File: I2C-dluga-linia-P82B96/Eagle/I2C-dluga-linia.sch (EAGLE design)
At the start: 15 parts

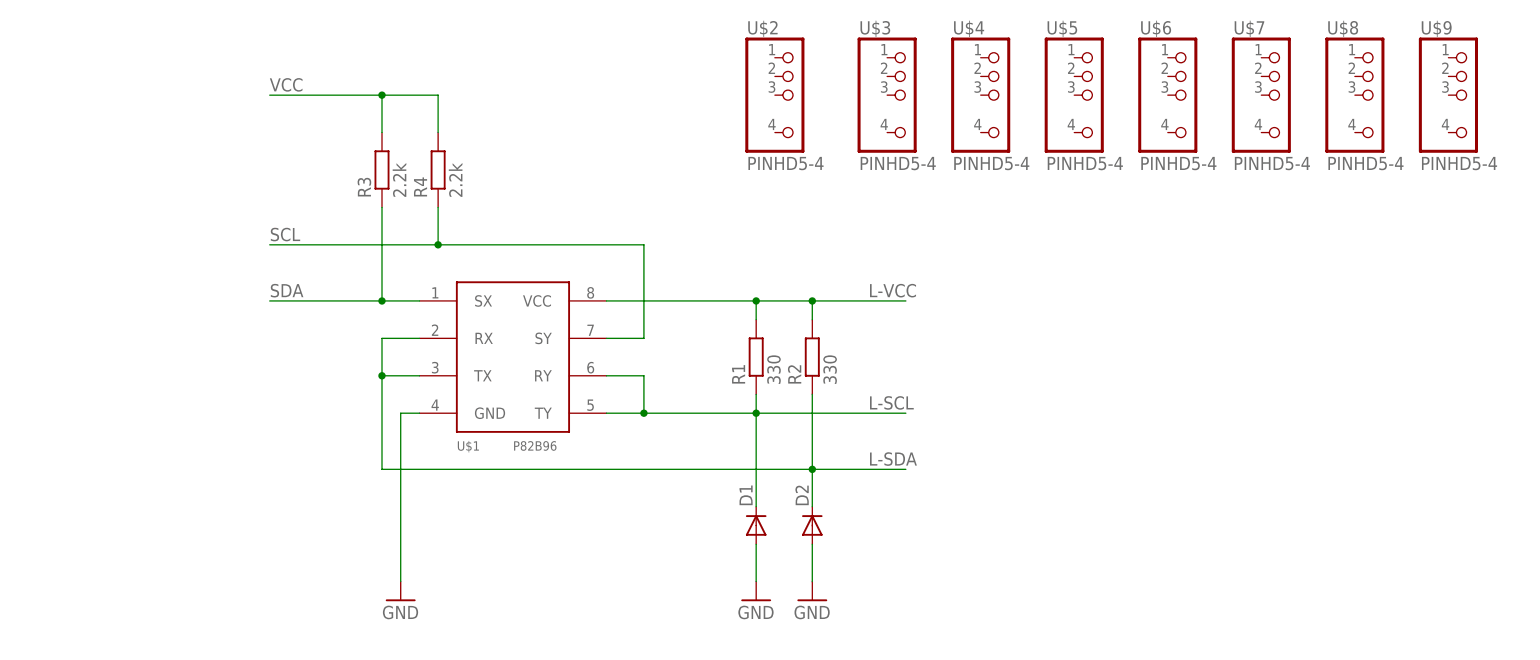
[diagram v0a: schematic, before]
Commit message: Podłączone złącza
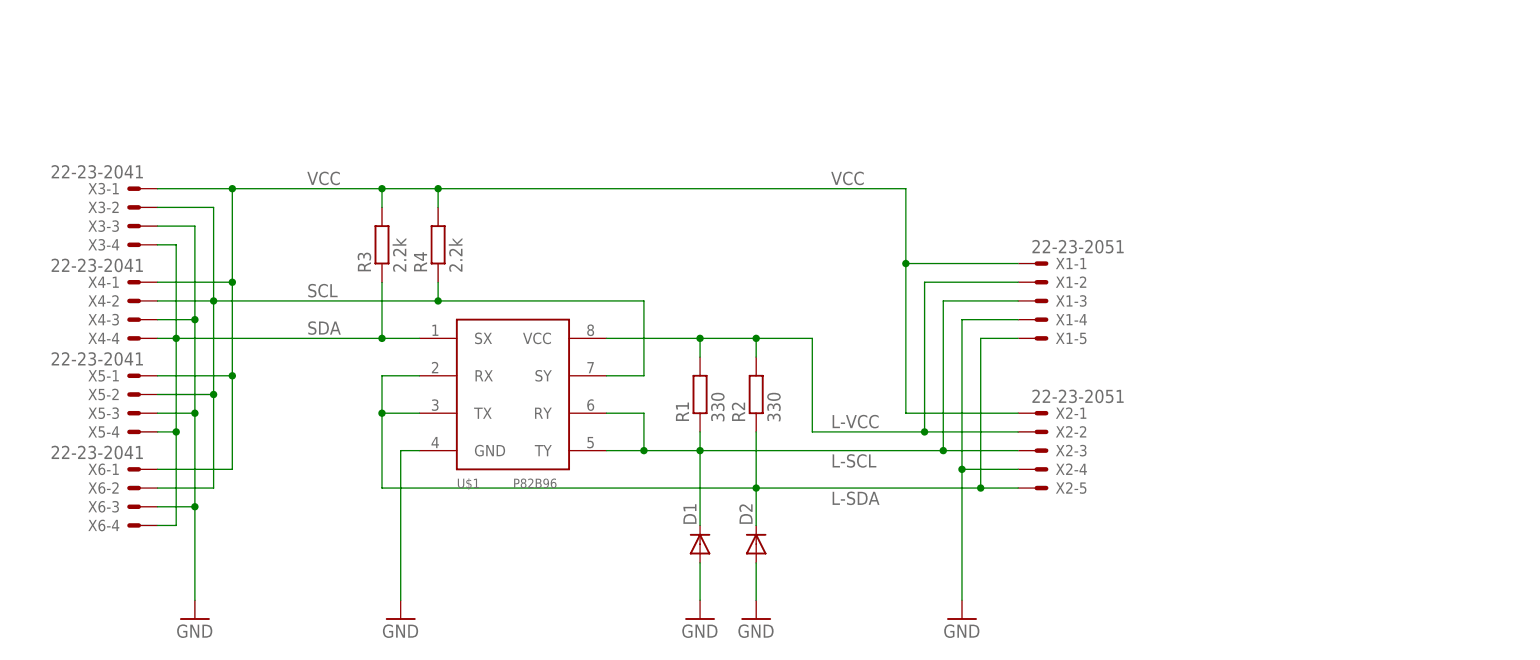
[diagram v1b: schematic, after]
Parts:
- removed U$2, U$3, U$4, U$5, U$6, U$7, U$8, U$9: PINHD5-4, RD:PINHD5-4
- added X1, X2: 22-23-2051, con-molex:22-23-2051
- added X3, X4, X5, X6: 22-23-2041, con-molex:22-23-2041
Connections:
- net GND: now also X1-4.S, X2-4.S, X3-3.S, X4-3.S, X5-3.S, X6-3.S
- net L-SCL: now also X1-3.S, X2-3.S
- net L-SDA: now also X1-5.S, X2-5.S
- net L-VCC: now also X1-2.S, X2-2.S
- net SCL: now also X3-2.S, X4-2.S, X5-2.S, X6-2.S
- net SDA: now also X3-4.S, X4-4.S, X5-4.S, X6-4.S
- net VCC: now also X1-1.S, X2-1.S, X3-1.S, X4-1.S, X5-1.S, X6-1.S
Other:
- moved on the sheet: D1, D2, R1, R2, R3, R4, U$1
